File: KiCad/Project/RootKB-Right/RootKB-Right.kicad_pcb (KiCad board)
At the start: 2 copper layers, 137.4 x 107.4 mm, 69 parts, among them J1 OLED-128x32, U1 Arduino_Pro_Micro, U2 TRRS

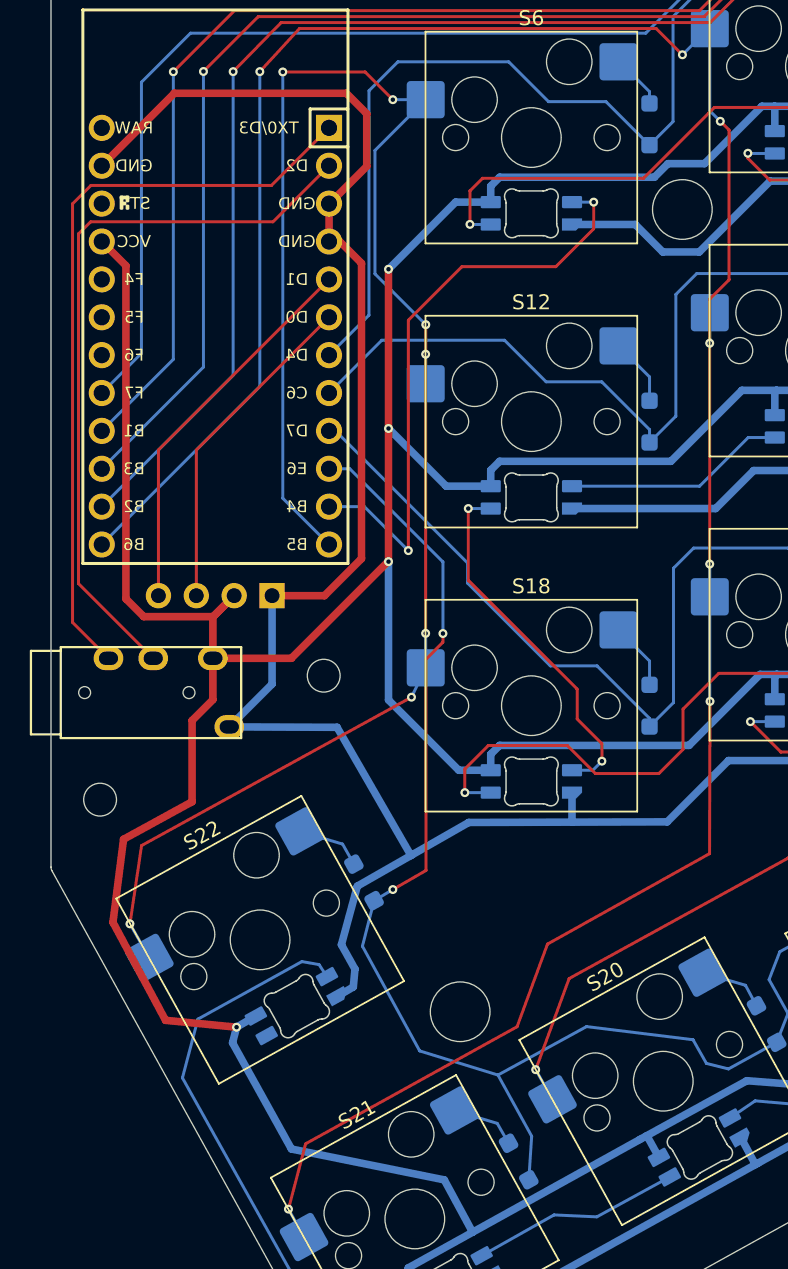
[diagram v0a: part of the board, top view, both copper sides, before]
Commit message: update routing
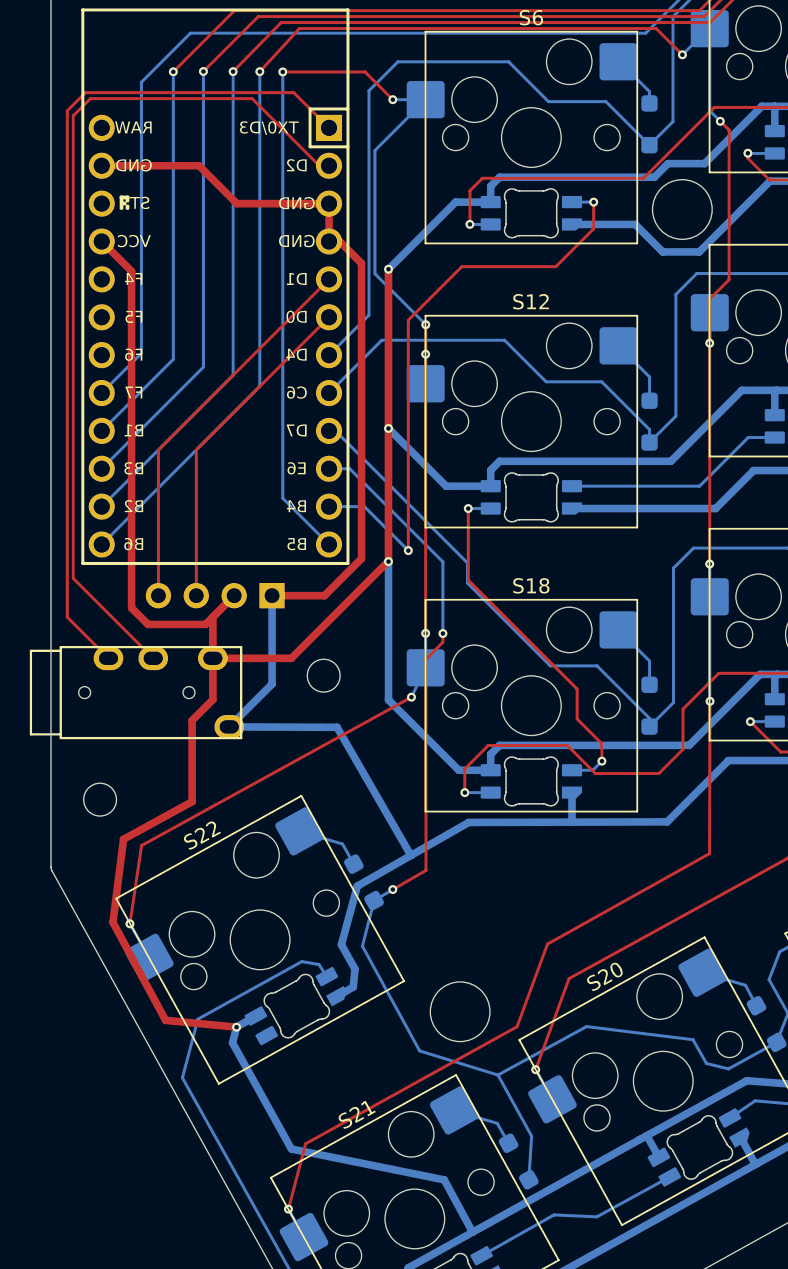
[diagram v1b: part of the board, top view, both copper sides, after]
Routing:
- net GND: track 576.3 -> 565.2 mm
- net TRRS_RX: track 49.2 -> 58.1 mm
- net TRRS_TX: track 50.8 -> 56.9 mm
- net VCC: track 551.4 -> 551.9 mm
